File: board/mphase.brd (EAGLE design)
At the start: 160 x 100 mm, 31 parts, among them IC1 MAX232, IC2 PIC18F4455_40, X1 332-10, X2 332-10

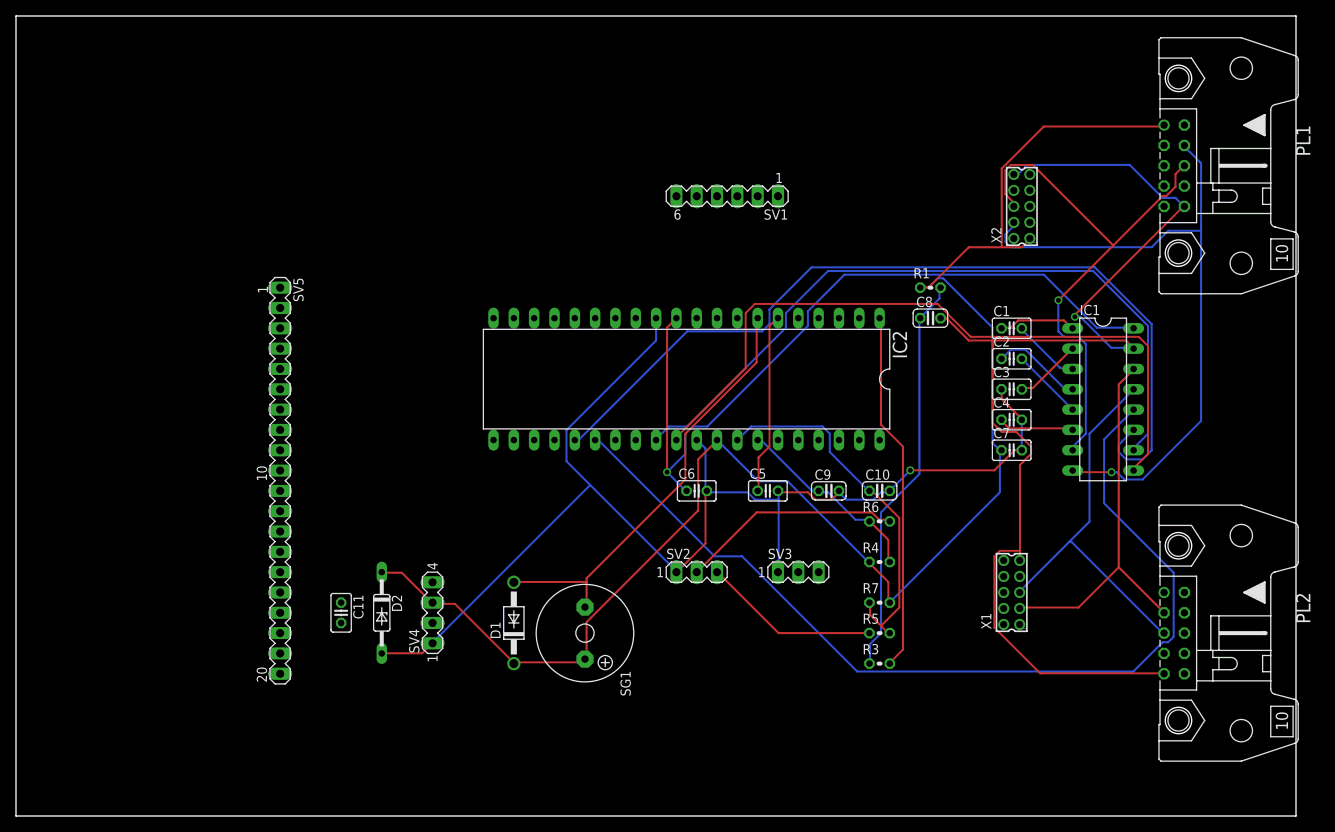
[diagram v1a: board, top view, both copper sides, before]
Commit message: updates
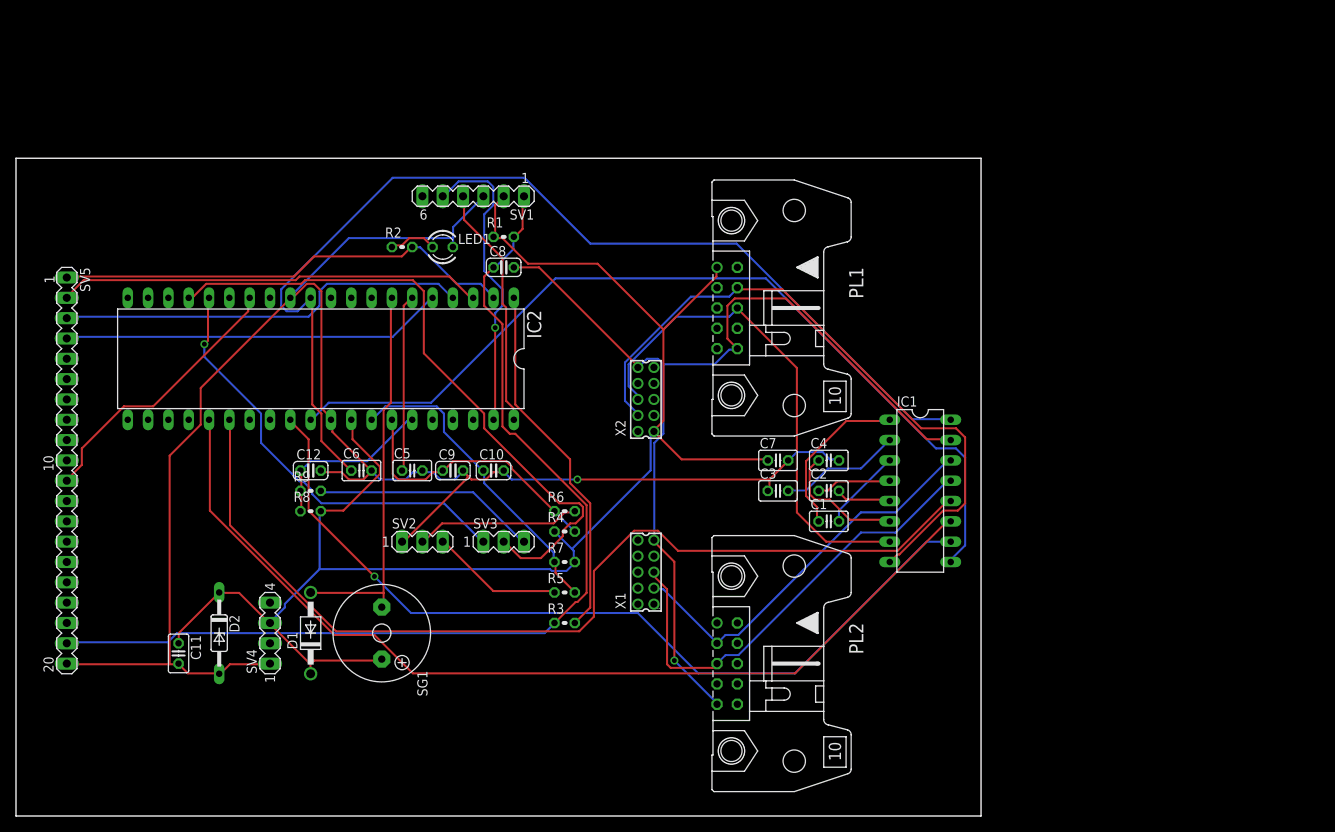
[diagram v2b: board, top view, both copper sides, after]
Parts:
- added C12: 0.1, resistor:C025-024X044
- added LED1: TLLR4400, led:LED3MM
- added R2, R9: 220, resistor:0204V
- added R8: 10000, resistor:0204V
- moved PL1 58.6 mm to (88.9, 63.5)
- moved PL2 56.0 mm to (88.9, 19.1)
- moved C8 53.7 mm to (61.0, 68.6)
- moved R1 53.7 mm to (61.0, 72.4)
- moved X2 52.8 mm to (78.7, 52.1)
- moved C10 48.3 mm to (59.7, 43.2)
- moved C9 47.1 mm to (54.6, 43.2)
- moved X1 45.8 mm to (78.7, 30.5)
- moved IC2 45.8 mm to (38.1, 57.1)
- moved C5 44.5 mm to (49.5, 43.2)
- moved C6 42.0 mm to (43.2, 43.2)
- moved R3 39.7 mm to (68.6, 24.1)
- moved R5 39.7 mm to (68.6, 27.9)
- moved R7 39.7 mm to (68.6, 31.8)
- moved R4 39.6 mm to (68.6, 35.6)
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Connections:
- new net N$15: IC2.2, R2.2, SV5.1
- new net N$18: LED1.A, R2.1
- new net N$23: IC2.3, SV5.2
- new net N$26: IC2.4, SV5.3
- new net N$27: IC2.5, SV5.4
- new net N$28: C12.1, IC2.35, R8.1, R9.1
- new net N$29: IC2.40, SV1.4
- new net N$30: IC2.14, SV5.11
- new net N$31: R9.2, SV3.3
- new net N$32: IC2.39, SV1.5
- new net N$33: IC2.16, SV3.1
- new net N$34: IC2.17, SV3.2
- net N$8: now also SV1.1, SV5.19
- net VDD: now also R8.2, SV1.2
- net VSS: now also C12.2, LED1.K, SV1.3, SV5.20; no longer SV3.1
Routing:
- net N$34: track 0.00 -> 82.0 mm
- net N$8: track 50.7 -> 125.1 mm
- net VSS: track 158.6 -> 224.9 mm
- net N$15: track 0.00 -> 57.6 mm
- net N$33: track 0.00 -> 54.5 mm, vias 0 -> 1
- net N$23: track 0.00 -> 53.1 mm
- net N$26: track 0.00 -> 51.9 mm
- net N$27: track 0.00 -> 47.9 mm
- net N$32: track 0.00 -> 38.4 mm, vias 0 -> 1
- net VCC: track 97.0 -> 132.5 mm, vias 1 -> 0
- net N$30: track 0.00 -> 34.5 mm
- net N$29: track 0.00 -> 30.5 mm
- net N$31: track 0.00 -> 28.1 mm
- net N$13: track 88.9 -> 112.3 mm
- net GND: track 145.3 -> 122.5 mm
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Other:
- board size 160 x 100 mm -> 120.6 x 82.2 mm
